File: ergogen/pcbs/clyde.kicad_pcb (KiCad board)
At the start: 2 copper layers, 114.3 x 82.4 mm, 24 parts

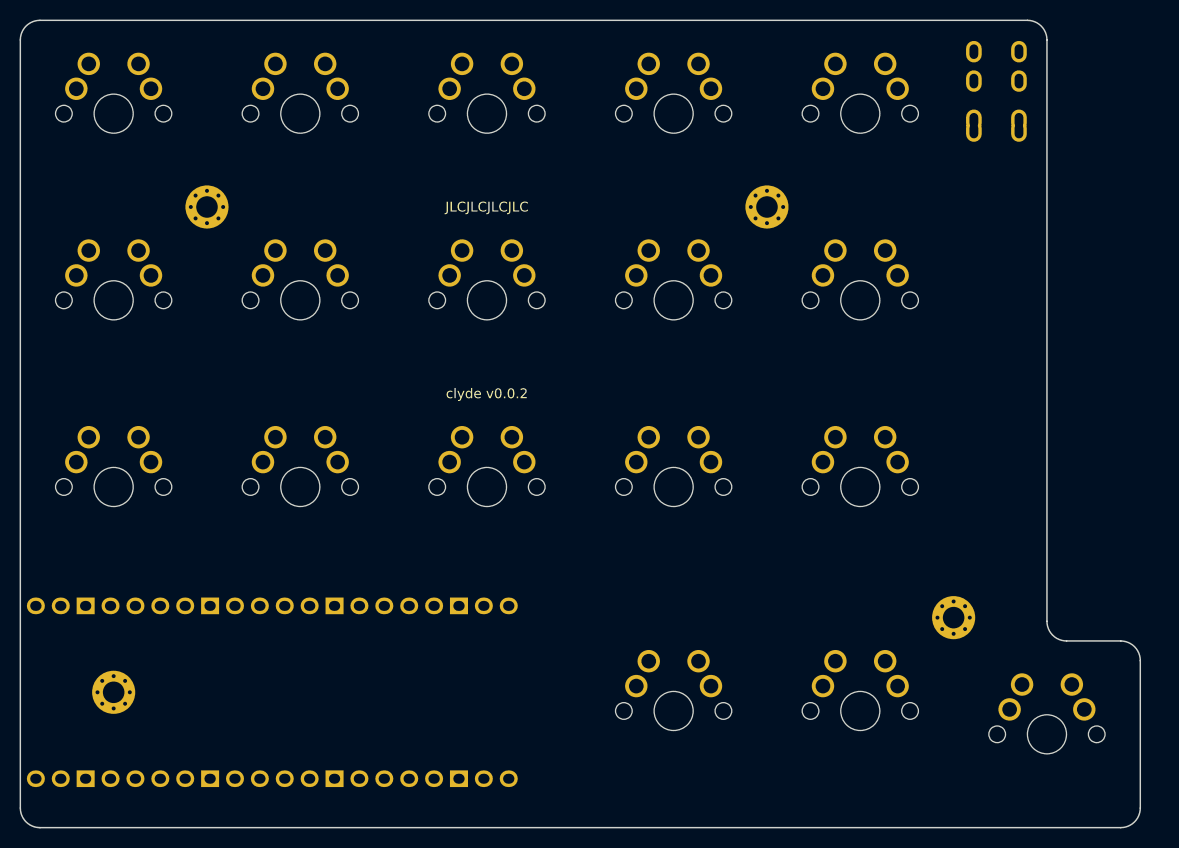
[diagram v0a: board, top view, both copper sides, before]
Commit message: begin work on v1
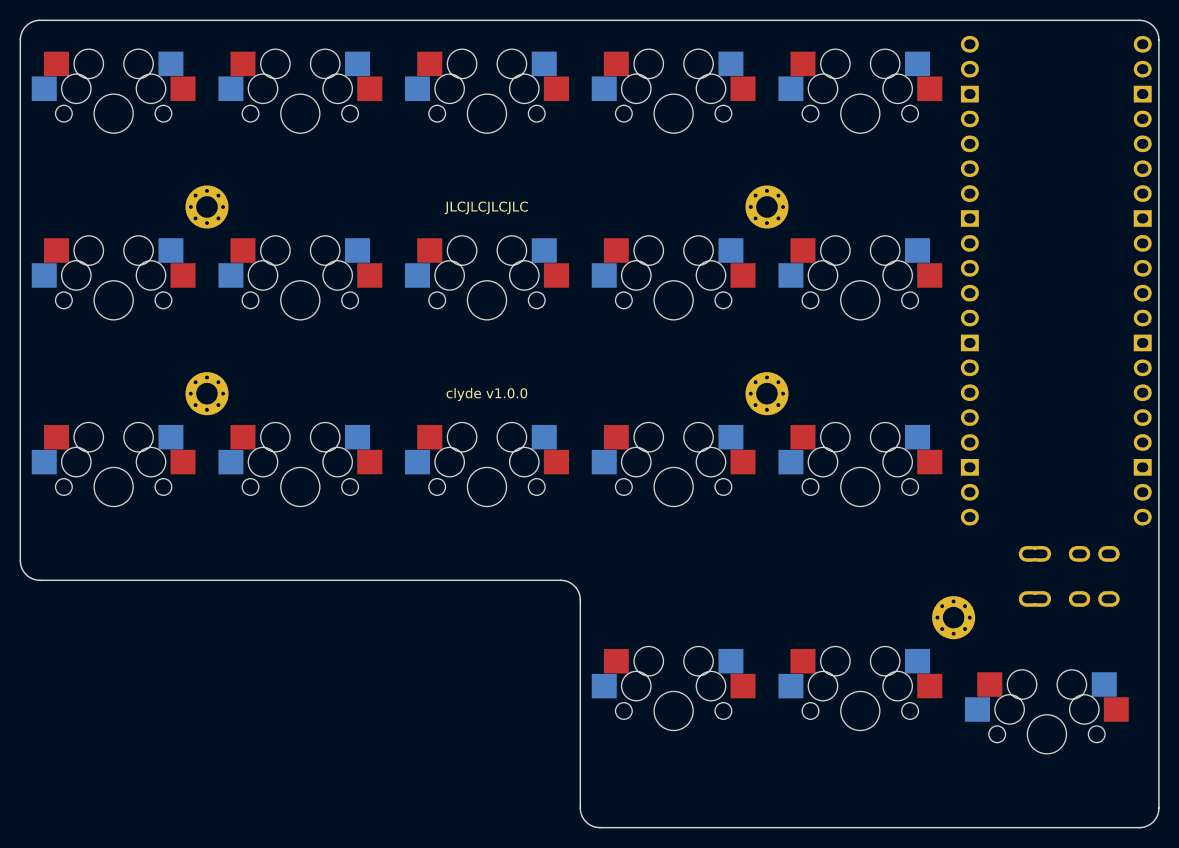
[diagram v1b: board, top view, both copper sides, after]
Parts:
- added _8: , MountingHole_2.2mm_M2_Pad_Via, F.Cu at (219.1, 142.9)
- U0: footprint RPi_Pico_TH_oval_face_down -> RPi_Pico_TH_oval_face_up
- moved U0 90.4 mm to (248.6, 131.3), turned to 0 degrees
- moved TRRS1 60.3 mm to (257.2, 163.8), turned to 270 degrees
- moved _5 50.4 mm to (161.9, 123.8)
- moved _6 19.1 mm to (161.9, 142.9)
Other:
- board size 114.3 x 82.4 mm -> 116.2 x 82.4 mm
- board text added: "clyde v1.0.0"
- board text removed: "clyde v0.0.2"
